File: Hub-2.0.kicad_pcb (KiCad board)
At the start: 2 copper layers, 149.2 x 100 mm, 41 parts, among them CN4 DT15-12PA, CN5 DT15-12PA, CN6 DT15-12PA, J10-PCB1 5569-16A2, J2-PCB1 5569-20A2, J3-PCB1 5569-06A2, J4-PCB1 5569-08A2, J5-PCB1 5569-18A2

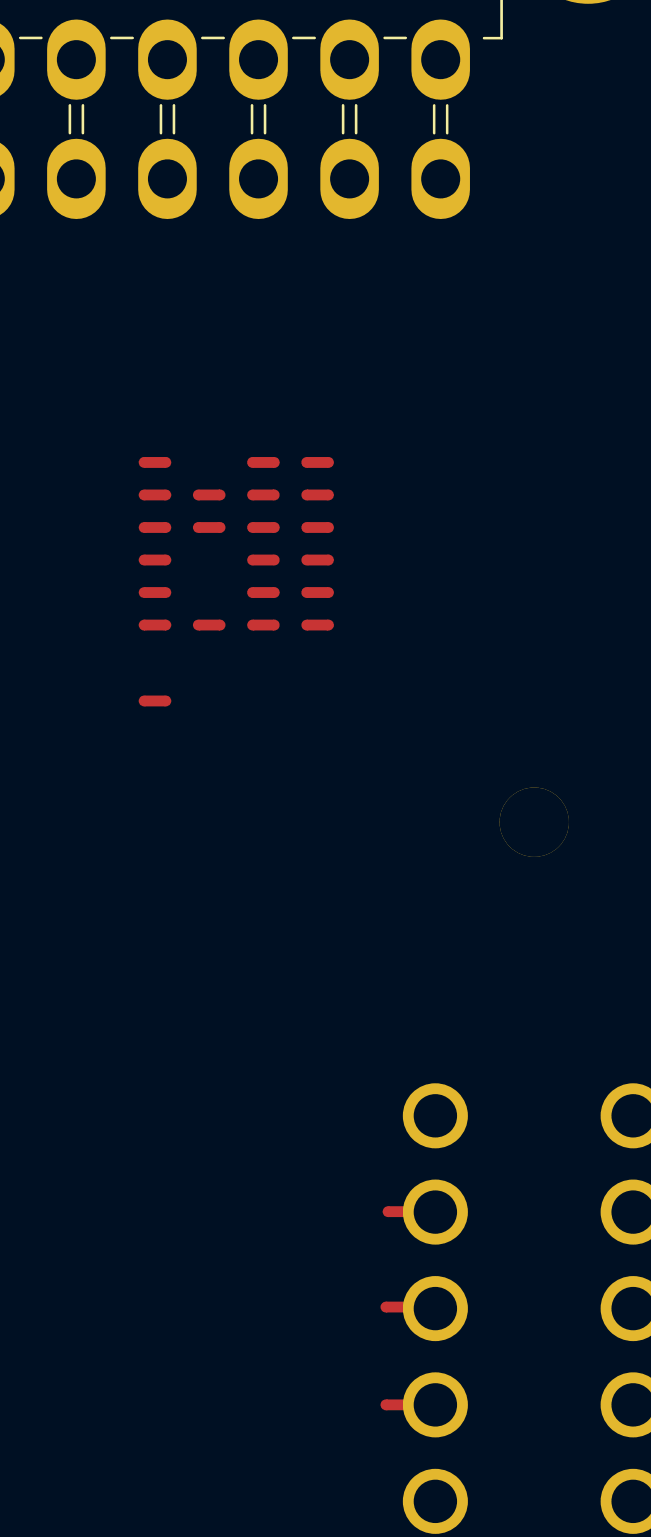
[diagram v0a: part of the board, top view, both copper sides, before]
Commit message: Autosave
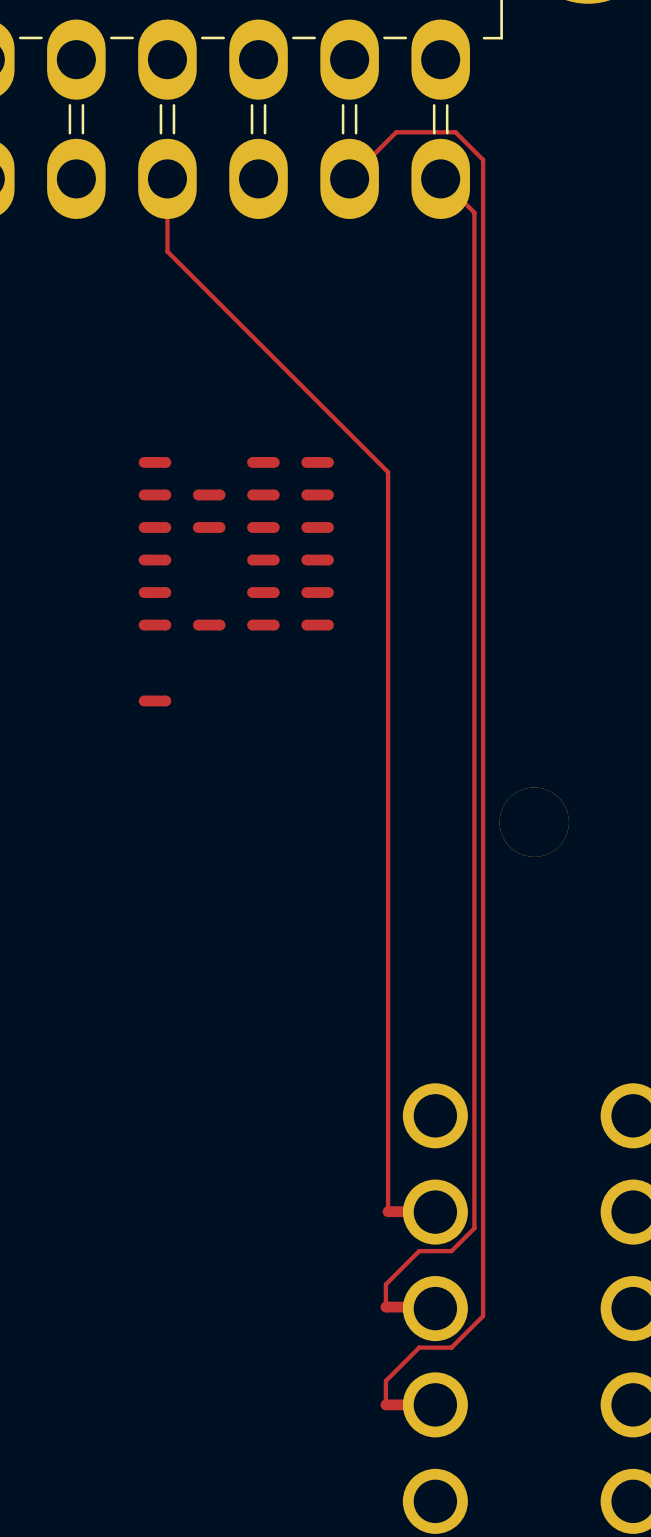
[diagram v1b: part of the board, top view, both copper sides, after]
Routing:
- net /ECU_INTERFACE/ECU_IN_IAT: track 0.00 -> 67.7 mm
- net /ECU_INTERFACE/ECU_IN_CLT: track 0.00 -> 55.2 mm
- net /ECU_INTERFACE/ECU_IN_TPS1: track 0.00 -> 51.8 mm
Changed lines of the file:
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@@
 		(layer "User.4")
+	)
+	(segment
+		(start 127.700001 87.8)
+		(end 127.700001 53.700001)
+		(width 0.2)
+		(layer "F.Cu")
+		(net "/ECU_INTERFACE/ECU_IN_TPS1")
+	)
+	(segment
+		(start 117.525001 43.525001)
+		(end 117.525001 40.175)
+		(width 0.2)
+		(layer "F.Cu")
+		(net "/ECU_INTERFACE/ECU_IN_TPS1")
+	)
+	(segment
+		(start 127.700001 53.700001)
+		(end 117.525001 43.525001)
+		(width 0.2)
+		(layer "F.Cu")
+		(net "/ECU_INTERFACE/ECU_IN_TPS1")
+	)
+	(segment
+		(start 127.600002 95.604413)
+		(end 129.134415 94.07)
+		(width 0.2)
+		(layer "F.Cu")
+		(net "/ECU_INTERFACE/ECU_IN_IAT")
+	)
+	(segment
+		(start 130.625585 94.07)
+		(end 132.08 92.615585)
+		(width 0.2)
+		(layer "F.Cu")
+		(net "/ECU_INTERFACE/ECU_IN_IAT")
+	)
+	(segment
+		(start 129.134415 94.07)
+		(end 130.625585 94.07)
+		(width 0.2)
+		(layer "F.Cu")
+		(net "/ECU_INTERFACE/ECU_IN_IAT")
+	)
+	(segment
+		(start 130.808453 38.025)
+		(end 128.075001 38.025)
+		(width 0.2)
+		(layer "F.Cu")
+		(net "/ECU_INTERFACE/ECU_IN_IAT")
+	)
+	(segment
+		(start 128.075001 38.025)
+		(end 125.925001 40.175)
+		(width 0.2)
+		(layer "F.Cu")
+		(net "/ECU_INTERFACE/ECU_IN_IAT")
+	)
+	(segment
+		(start 132.08 39.296547)
+		(end 130.808453 38.025)
+		(width 0.2)
+		(layer "F.Cu")
+		(net "/ECU_INTERFACE/ECU_IN_IAT")
+	)
+	(segment
+		(start 127.600002 96.71)
+		(end 127.600002 95.604413)
+		(width 0.2)
+		(layer "F.Cu")
+		(net "/ECU_INTERFACE/ECU_IN_IAT")
+	)
+	(segment
+		(start 132.08 92.615585)
+		(end 132.08 39.296547)
+		(width 0.2)
+		(layer "F.Cu")
+		(net "/ECU_INTERFACE/ECU_IN_IAT")
+	)
+	(segment
+		(start 129.134415 89.62)
+		(end 130.625585 89.62)
+		(width 0.2)
+		(layer "F.Cu")
+		(net "/ECU_INTERFACE/ECU_IN_CLT")
+	)
+	(segment
+		(start 127.600001 91.154414)
+		(end 129.134415 89.62)
+		(width 0.2)
+		(layer "F.Cu")
+		(net "/ECU_INTERFACE/ECU_IN_CLT")
+	)
+	(segment
+		(start 131.68 88.565585)
+		(end 131.68 41.729999)
+		(width 0.2)
+		(layer "F.Cu")
+		(net "/ECU_INTERFACE/ECU_IN_CLT")
+	)
+	(segment
+		(start 131.68 41.729999)
+		(end 130.125001 40.175)
+		(width 0.2)
+		(layer "F.Cu")
+		(net "/ECU_INTERFACE/ECU_IN_CLT")
+	)
+	(segment
+		(start 130.625585 89.62)
+		(end 131.68 88.565585)
+		(width 0.2)
+		(layer "F.Cu")
+		(net "/ECU_INTERFACE/ECU_IN_CLT")
+	)
+	(segment
+		(start 127.600001 92.2)
+		(end 127.600001 91.154414)
+		(width 0.2)
+		(layer "F.Cu")
+		(net "/ECU_INTERFACE/ECU_IN_CLT")
 	)
 	(embedded_fonts no)

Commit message: SCH Save
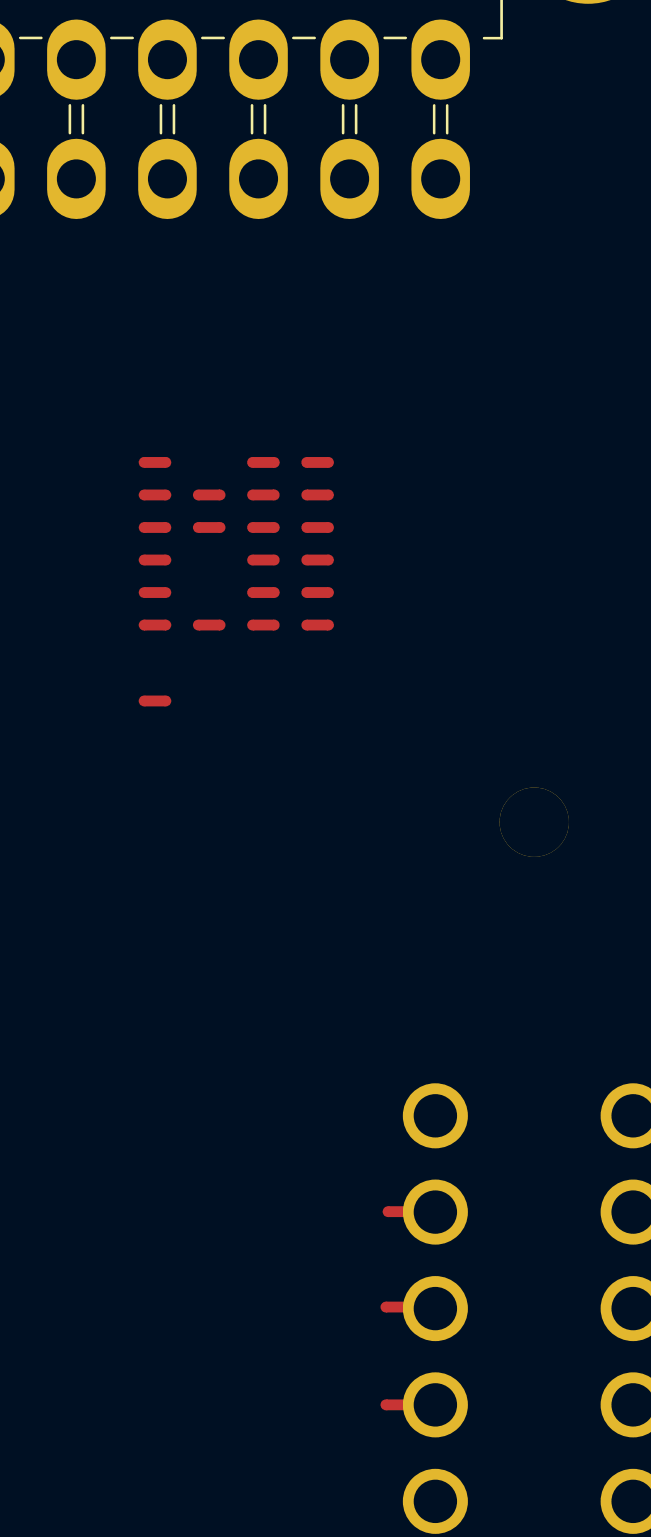
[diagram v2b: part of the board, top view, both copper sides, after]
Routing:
- net /ECU_INTERFACE/ECU_IN_IAT: track 67.7 -> 0.00 mm
- net /ECU_INTERFACE/ECU_IN_CLT: track 55.2 -> 0.00 mm
- net /ECU_INTERFACE/ECU_IN_TPS1: track 51.8 -> 0.00 mm
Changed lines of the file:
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@@
 		(layer "User.4")
-	)
-	(segment
-		(start 127.700001 87.8)
-		(end 127.700001 53.700001)
-		(width 0.2)
-		(layer "F.Cu")
-		(net "/ECU_INTERFACE/ECU_IN_TPS1")
-	)
-	(segment
-		(start 117.525001 43.525001)
-		(end 117.525001 40.175)
-		(width 0.2)
-		(layer "F.Cu")
-		(net "/ECU_INTERFACE/ECU_IN_TPS1")
-	)
-	(segment
-		(start 127.700001 53.700001)
-		(end 117.525001 43.525001)
-		(width 0.2)
-		(layer "F.Cu")
-		(net "/ECU_INTERFACE/ECU_IN_TPS1")
-	)
-	(segment
-		(start 127.600002 95.604413)
-		(end 129.134415 94.07)
-		(width 0.2)
-		(layer "F.Cu")
-		(net "/ECU_INTERFACE/ECU_IN_IAT")
-	)
-	(segment
-		(start 130.625585 94.07)
-		(end 132.08 92.615585)
-		(width 0.2)
-		(layer "F.Cu")
-		(net "/ECU_INTERFACE/ECU_IN_IAT")
-	)
-	(segment
-		(start 129.134415 94.07)
-		(end 130.625585 94.07)
-		(width 0.2)
-		(layer "F.Cu")
-		(net "/ECU_INTERFACE/ECU_IN_IAT")
-	)
-	(segment
-		(start 130.808453 38.025)
-		(end 128.075001 38.025)
-		(width 0.2)
-		(layer "F.Cu")
-		(net "/ECU_INTERFACE/ECU_IN_IAT")
-	)
-	(segment
-		(start 128.075001 38.025)
-		(end 125.925001 40.175)
-		(width 0.2)
-		(layer "F.Cu")
-		(net "/ECU_INTERFACE/ECU_IN_IAT")
-	)
-	(segment
-		(start 132.08 39.296547)
-		(end 130.808453 38.025)
-		(width 0.2)
-		(layer "F.Cu")
-		(net "/ECU_INTERFACE/ECU_IN_IAT")
-	)
-	(segment
-		(start 127.600002 96.71)
-		(end 127.600002 95.604413)
-		(width 0.2)
-		(layer "F.Cu")
-		(net "/ECU_INTERFACE/ECU_IN_IAT")
-	)
-	(segment
-		(start 132.08 92.615585)
-		(end 132.08 39.296547)
-		(width 0.2)
-		(layer "F.Cu")
-		(net "/ECU_INTERFACE/ECU_IN_IAT")
-	)
-	(segment
-		(start 129.134415 89.62)
-		(end 130.625585 89.62)
-		(width 0.2)
-		(layer "F.Cu")
-		(net "/ECU_INTERFACE/ECU_IN_CLT")
-	)
-	(segment
-		(start 127.600001 91.154414)
-		(end 129.134415 89.62)
-		(width 0.2)
-		(layer "F.Cu")
-		(net "/ECU_INTERFACE/ECU_IN_CLT")
-	)
-	(segment
-		(start 131.68 88.565585)
-		(end 131.68 41.729999)
-		(width 0.2)
-		(layer "F.Cu")
-		(net "/ECU_INTERFACE/ECU_IN_CLT")
-	)
-	(segment
-		(start 131.68 41.729999)
-		(end 130.125001 40.175)
-		(width 0.2)
-		(layer "F.Cu")
-		(net "/ECU_INTERFACE/ECU_IN_CLT")
-	)
-	(segment
-		(start 130.625585 89.62)
-		(end 131.68 88.565585)
-		(width 0.2)
-		(layer "F.Cu")
-		(net "/ECU_INTERFACE/ECU_IN_CLT")
-	)
-	(segment
-		(start 127.600001 92.2)
-		(end 127.600001 91.154414)
-		(width 0.2)
-		(layer "F.Cu")
-		(net "/ECU_INTERFACE/ECU_IN_CLT")
 	)
 	(embedded_fonts no)
